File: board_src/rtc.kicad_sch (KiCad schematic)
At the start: 8 parts, among them IC1 PCF8563TS_4,118, J9 Conn_01x02_Pin, Y2 Crystal

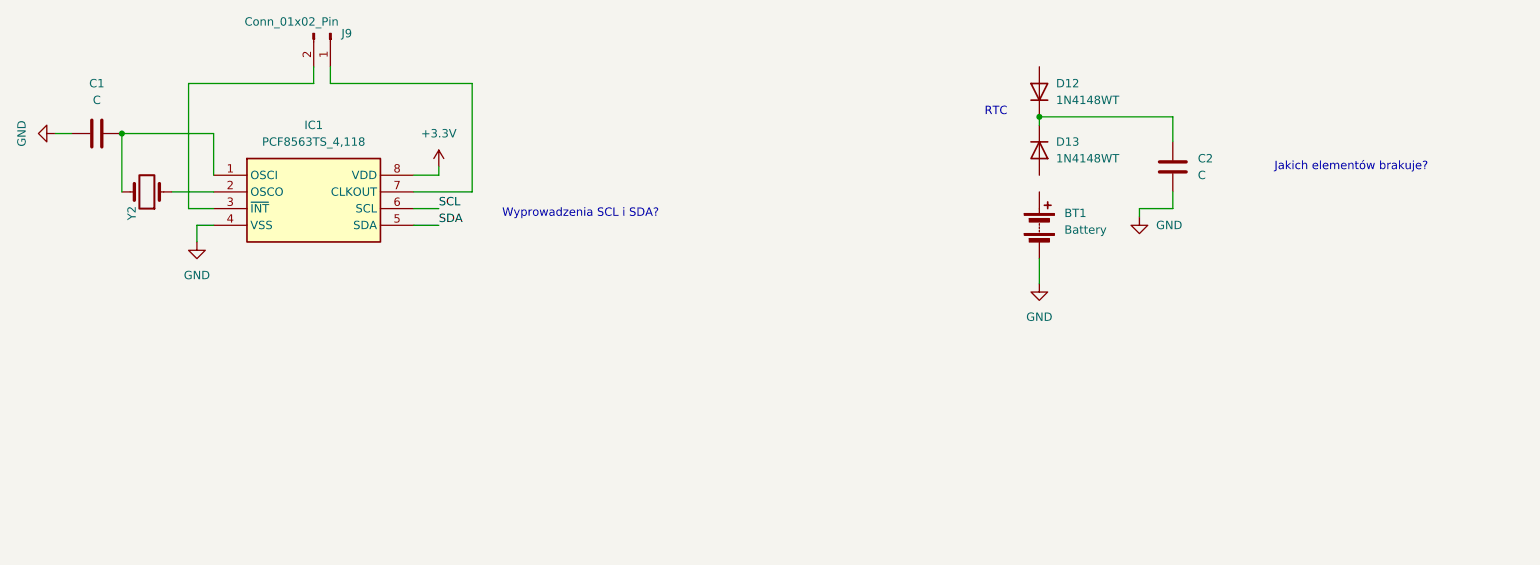
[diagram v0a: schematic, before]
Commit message: wersja dodane arkusze hierarchiczne
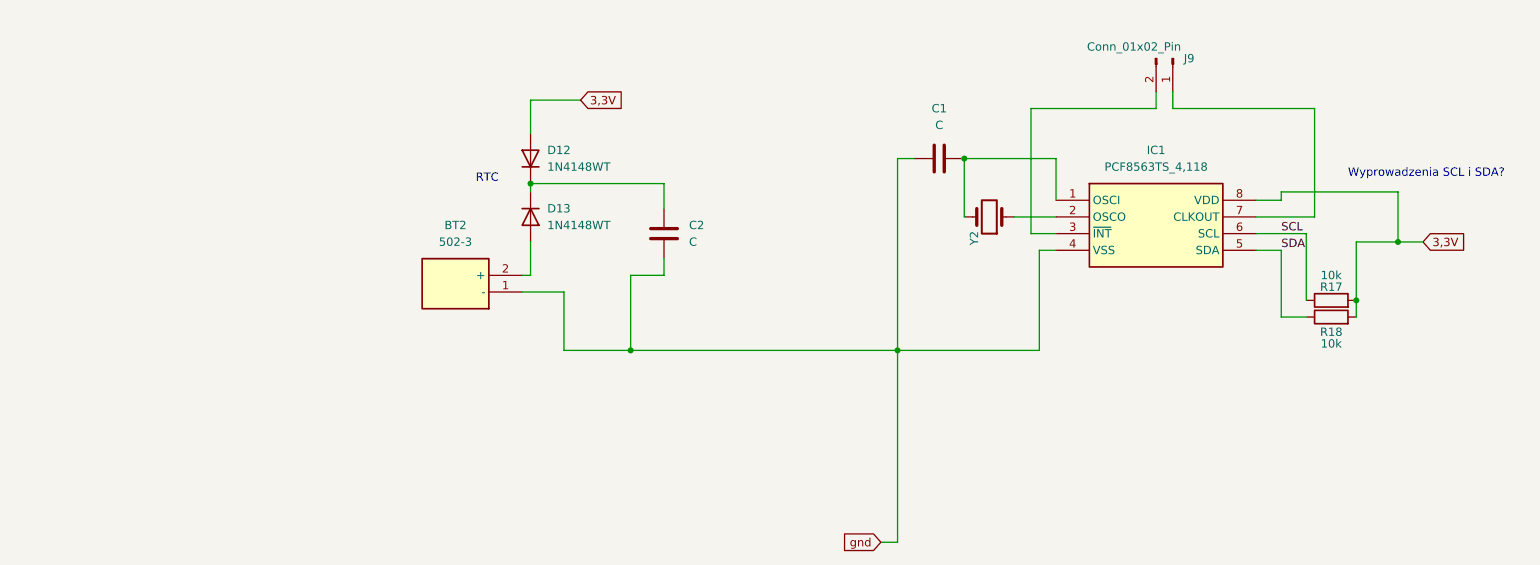
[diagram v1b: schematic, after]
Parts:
- removed BT1: Battery, symbol Device:Battery
- added BT2: 502-3, 5023, symbol 502-3:502-3
- added R17, R18: 10k, Resistor_SMD:R_0201_0603Metric, symbol Device:R
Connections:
- net +3.3V is gone; now on net 3,3V: IC1.8 (VDD)
- net SCL: now also R17.1
- net SDA: now also R18.1
- net at D13.2 (A): now also BT2.2 (+)
- net 3,3V: now reaches D12.2 (A)
- net 3,3V: now also R17.2, R18.2
- net GND renamed gnd
- net gnd: now also BT2.1 (-)
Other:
- note removed: "Jakich elementów brakuje?"
- moved on the sheet: C1, C2, D12, D13, IC1, J9, Y2
